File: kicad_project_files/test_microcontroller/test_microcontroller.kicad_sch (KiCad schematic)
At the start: 40 parts, among them J1 USB4510-03-1-A_REVA, SW1 SW_Push, SW2 SW_Push, SW3 SW_Push, SW4 SW_Push, SW5 SW_Push, SW6 SW_Push, SW7 SW_Push, SW8 SW_Push, SW9 SW_Push, U1 ATmega8U2-A, Y1 16mhz

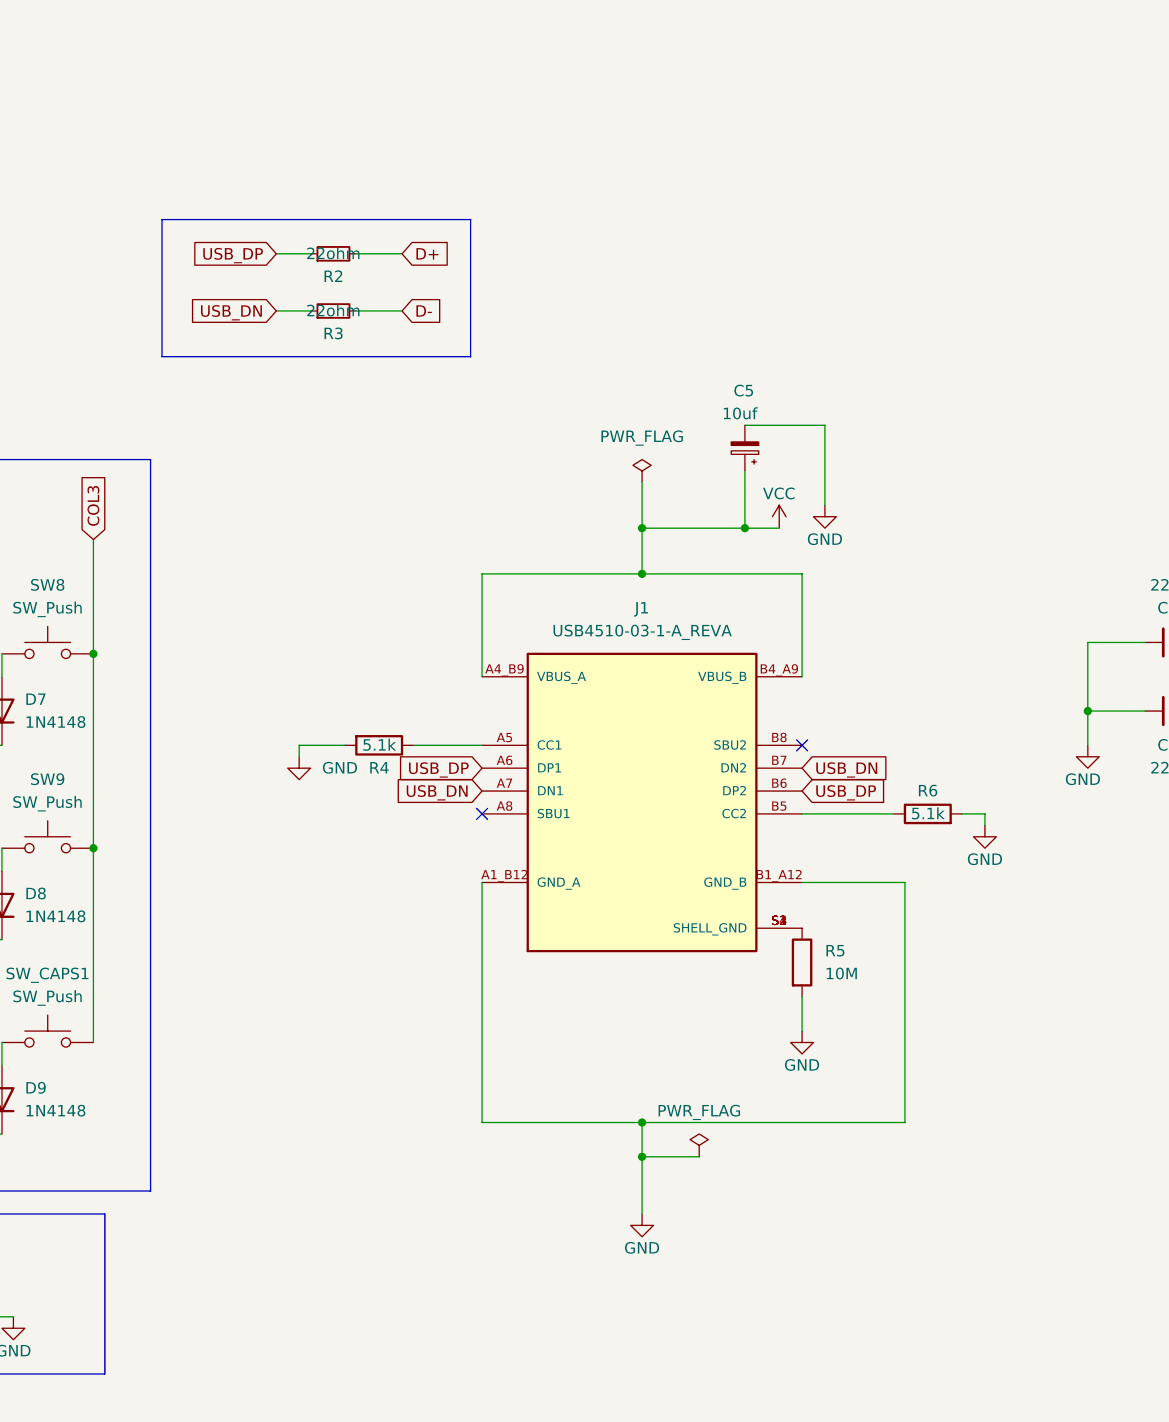
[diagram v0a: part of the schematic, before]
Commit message: Revert "Revert "Merge branch 'main' of https://github.com/Goochy12/Keych-and-Chong""
This reverts commit c8ae18377c4835621f54e74df08cb33c8008ec0a.
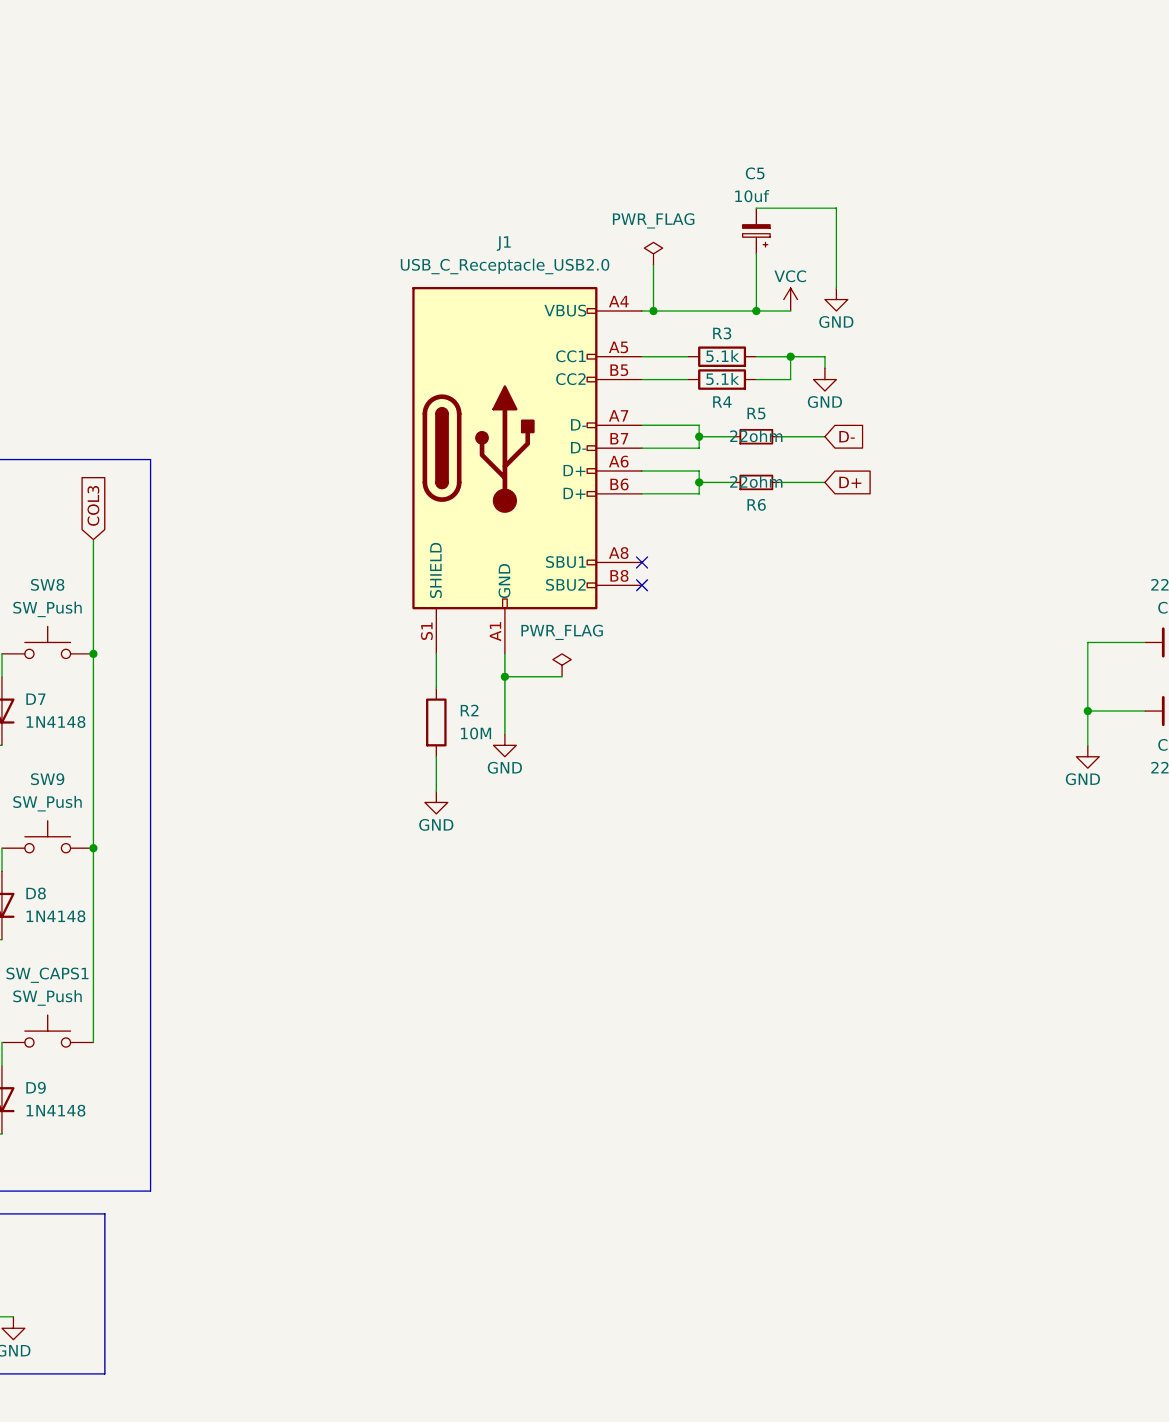
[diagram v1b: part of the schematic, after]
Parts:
- removed J1: USB4510-03-1-A_REVA, GCT_USB4510-03-1-A_REVA:GCT_USB4510-03-1-A_REVA, symbol USB4510-03-1-A_REVA:USB4510-03-1-A_REVA
- removed R2, R3: 22ohm, Resistor_THT:R_Axial_DIN0204_L3.6mm_D1.6mm_P5.08mm_Horizontal, symbol Device:R_Small
- removed R5: 10M, Resistor_THT:R_Axial_DIN0204_L3.6mm_D1.6mm_P5.08mm_Horizontal, symbol Device:R
- removed R6: 5.1k, Resistor_THT:R_Axial_DIN0204_L3.6mm_D1.6mm_P5.08mm_Horizontal, symbol Device:R
- added J1: USB_C_Receptacle_USB2.0, Connector_USB:USB_C_Receptacle_HRO_TYPE-C-31-M-12, symbol Connector:USB_C_Receptacle_USB2.0
- added R2: 10M, Resistor_THT:R_Axial_DIN0204_L3.6mm_D1.6mm_P5.08mm_Horizontal, symbol Device:R
- added R3: 5.1k, Resistor_THT:R_Axial_DIN0204_L3.6mm_D1.6mm_P5.08mm_Horizontal, symbol Device:R
- added R5, R6: 22ohm, Resistor_THT:R_Axial_DIN0204_L3.6mm_D1.6mm_P5.08mm_Horizontal, symbol Device:R_Small
- D_CAPS1: footprint CLA1A_SMD_LED:CLA1A-WKW-CXAYB153 -> LED_SMD:LED_Cree-PLCC4_3.2x2.8mm_CCW
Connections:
- net D+: now also R6.2
- net D-: now also R5.2
- net GND: now also J1.A1 (GND), J1.A12 (GND), J1.B1 (GND), J1.B12 (GND), R2.2, R3.2
- net VCC: now also J1.A4 (VBUS), J1.A9 (VBUS), J1.B4 (VBUS), J1.B9 (VBUS)
- net at R4.1: now also J1.B5 (CC2)
- new net: J1.A5 (CC1), R3.1
- new net: J1.A6 (D+), J1.B6 (D+), R6.1
- new net: J1.A7 (D-), J1.B7 (D-), R5.1
- new net: J1.S1 (SHIELD), R2.1

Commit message: Revert "Merge branch 'main' of https://github.com/Goochy12/Keych-and-Chong"
This reverts commit 16abbc7445c5651a73e155e9e96779087de1ba9e, reversing
changes made to 1815a7fd47ddf9f2f8e947e23bdaa21c8c5a7216.
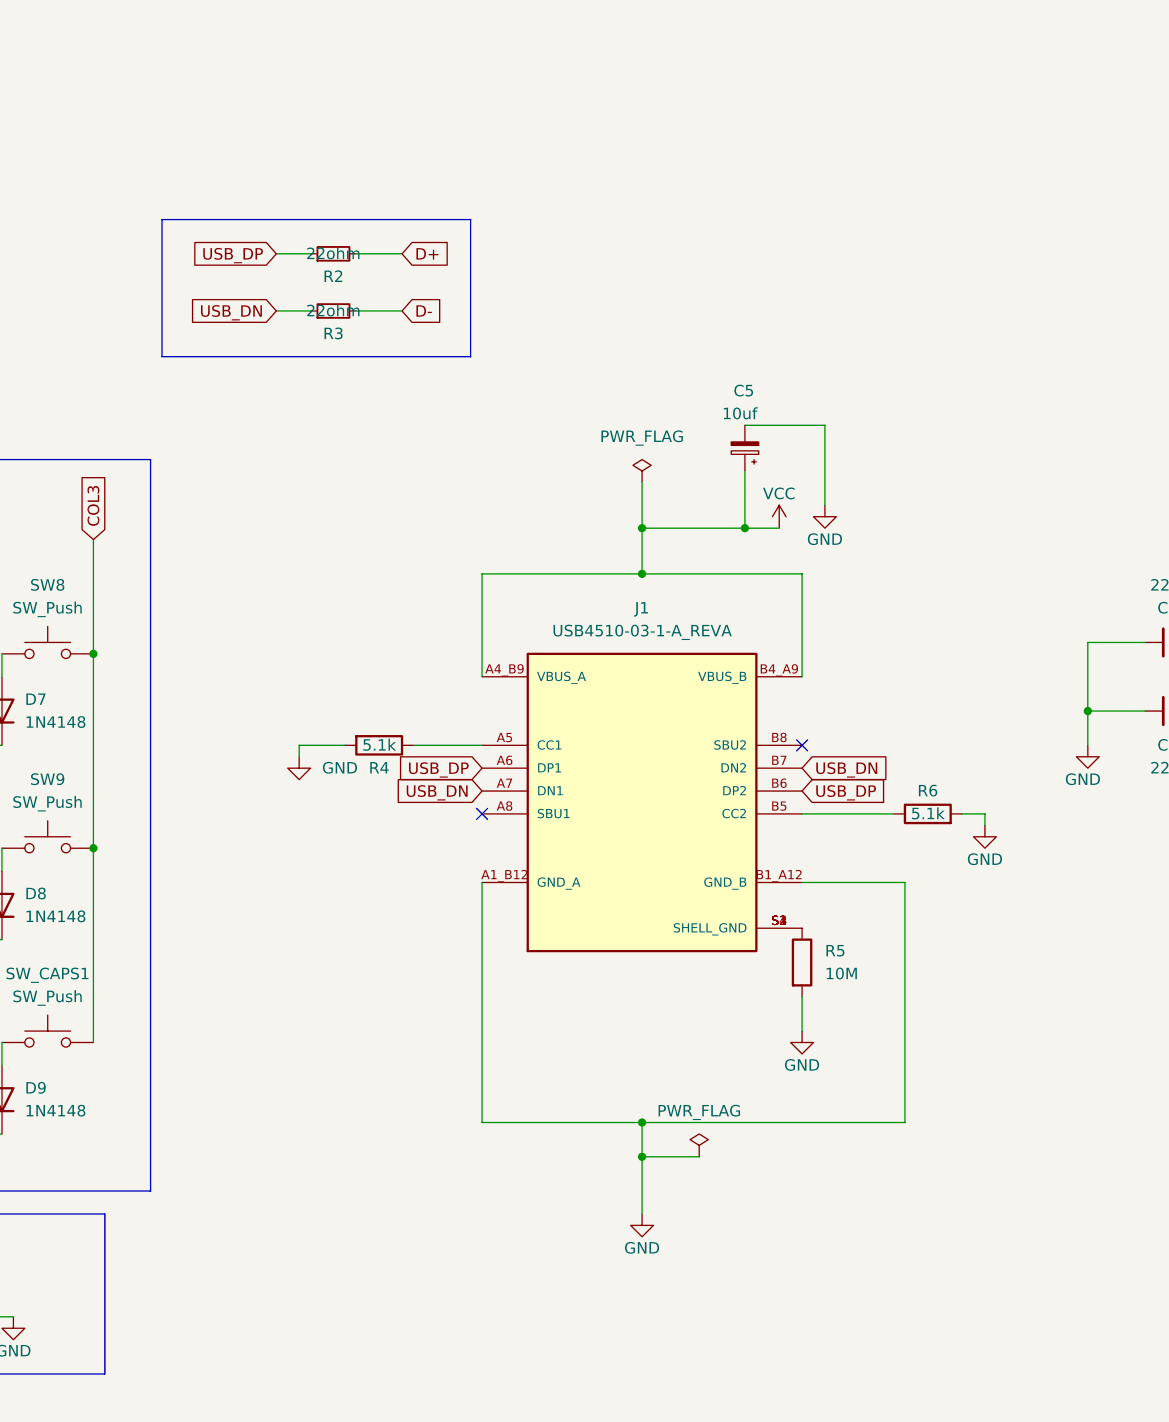
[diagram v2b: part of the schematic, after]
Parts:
- removed J1: USB_C_Receptacle_USB2.0, Connector_USB:USB_C_Receptacle_HRO_TYPE-C-31-M-12, symbol Connector:USB_C_Receptacle_USB2.0
- removed R2: 10M, Resistor_THT:R_Axial_DIN0204_L3.6mm_D1.6mm_P5.08mm_Horizontal, symbol Device:R
- removed R3: 5.1k, Resistor_THT:R_Axial_DIN0204_L3.6mm_D1.6mm_P5.08mm_Horizontal, symbol Device:R
- removed R5, R6: 22ohm, Resistor_THT:R_Axial_DIN0204_L3.6mm_D1.6mm_P5.08mm_Horizontal, symbol Device:R_Small
- added J1: USB4510-03-1-A_REVA, GCT_USB4510-03-1-A_REVA:GCT_USB4510-03-1-A_REVA, symbol USB4510-03-1-A_REVA:USB4510-03-1-A_REVA
- added R2, R3: 22ohm, Resistor_THT:R_Axial_DIN0204_L3.6mm_D1.6mm_P5.08mm_Horizontal, symbol Device:R_Small
- added R5: 10M, Resistor_THT:R_Axial_DIN0204_L3.6mm_D1.6mm_P5.08mm_Horizontal, symbol Device:R
- added R6: 5.1k, Resistor_THT:R_Axial_DIN0204_L3.6mm_D1.6mm_P5.08mm_Horizontal, symbol Device:R
- D_CAPS1: footprint LED_SMD:LED_Cree-PLCC4_3.2x2.8mm_CCW -> CLA1A_SMD_LED:CLA1A-WKW-CXAYB153
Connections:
- net D+: now also R2.2
- net D-: now also R3.2
- net GND: now also J1.A1_B12 (GND_A), J1.B1_A12 (GND_B), R5.2, R6.2
- net VCC: now also J1.A4_B9 (VBUS_A), J1.B4_A9 (VBUS_B)
- net at R4.1: now also J1.A5 (CC1)
- new net: J1.B5 (CC2), R6.1
- new net: J1.S1 (SHELL_GND), J1.S2 (SHELL_GND), J1.S3 (SHELL_GND), J1.S4 (SHELL_GND), R5.1
- new net USB_DN: J1.A7 (DN1), J1.B7 (DN2), R3.1
- new net USB_DP: J1.A6 (DP1), J1.B6 (DP2), R2.1

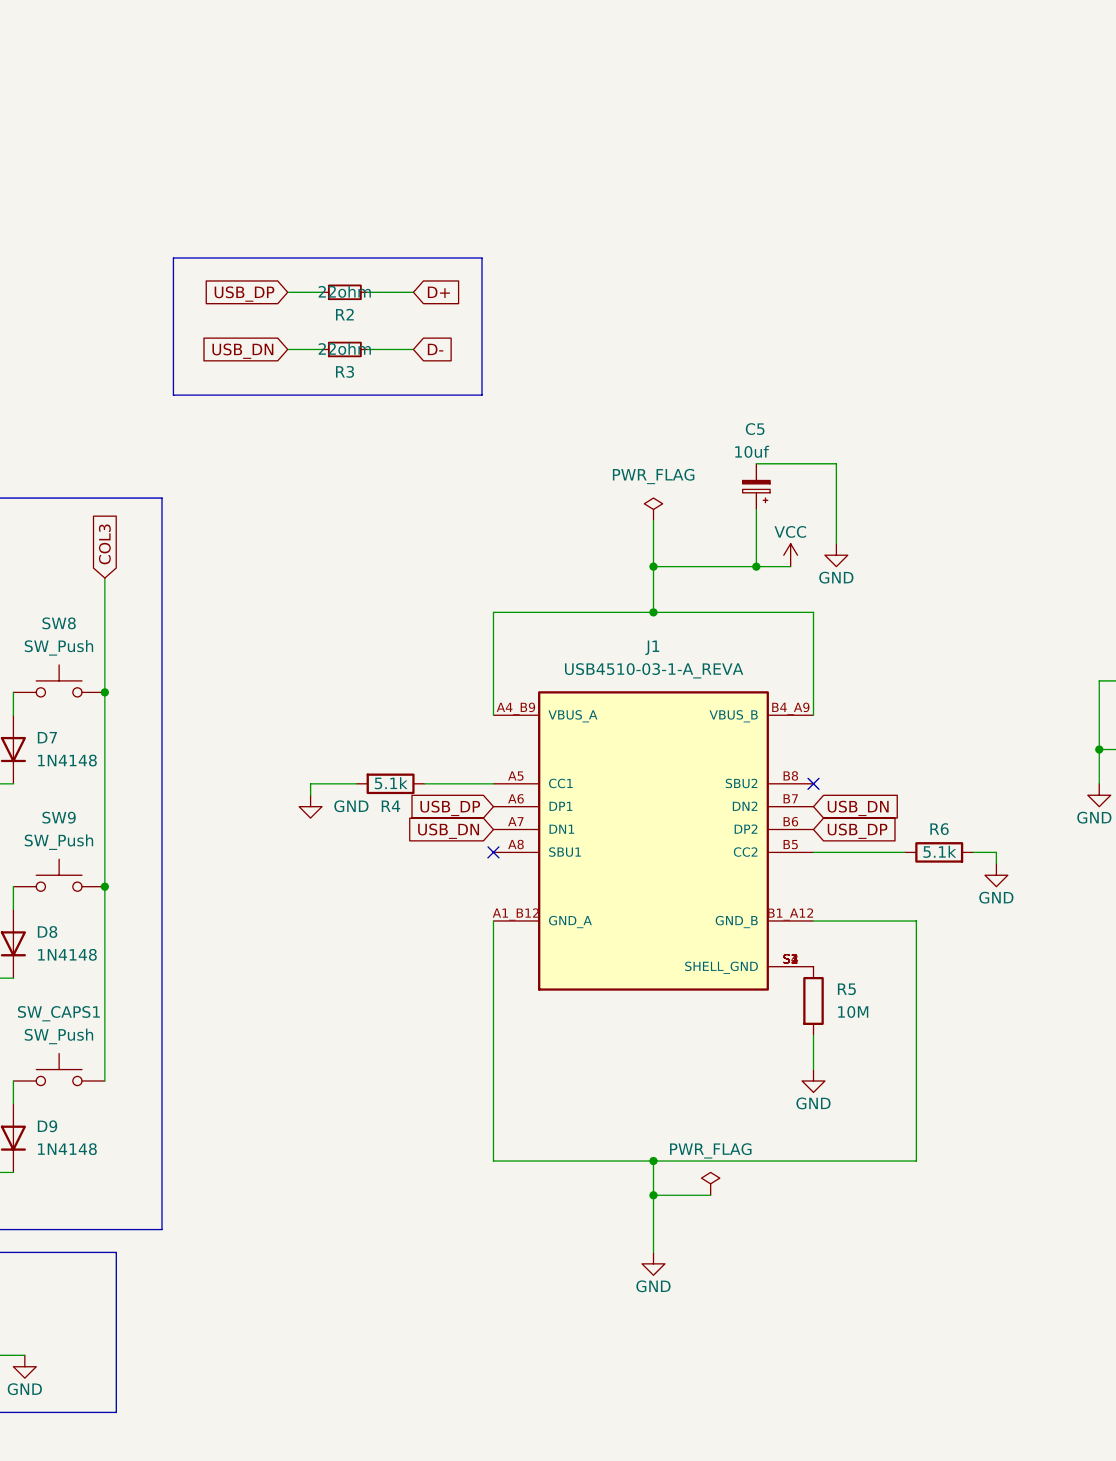
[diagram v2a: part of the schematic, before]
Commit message: Revert "Merge branch 'main' of https://github.com/Goochy12/Keych-and-Chong"
This reverts commit 89a84faf58301de3235cbf20de78d9bc04a2e137, reversing
changes made to 8f87e55d37906a6161fcb491ec761d32a82a7e61.
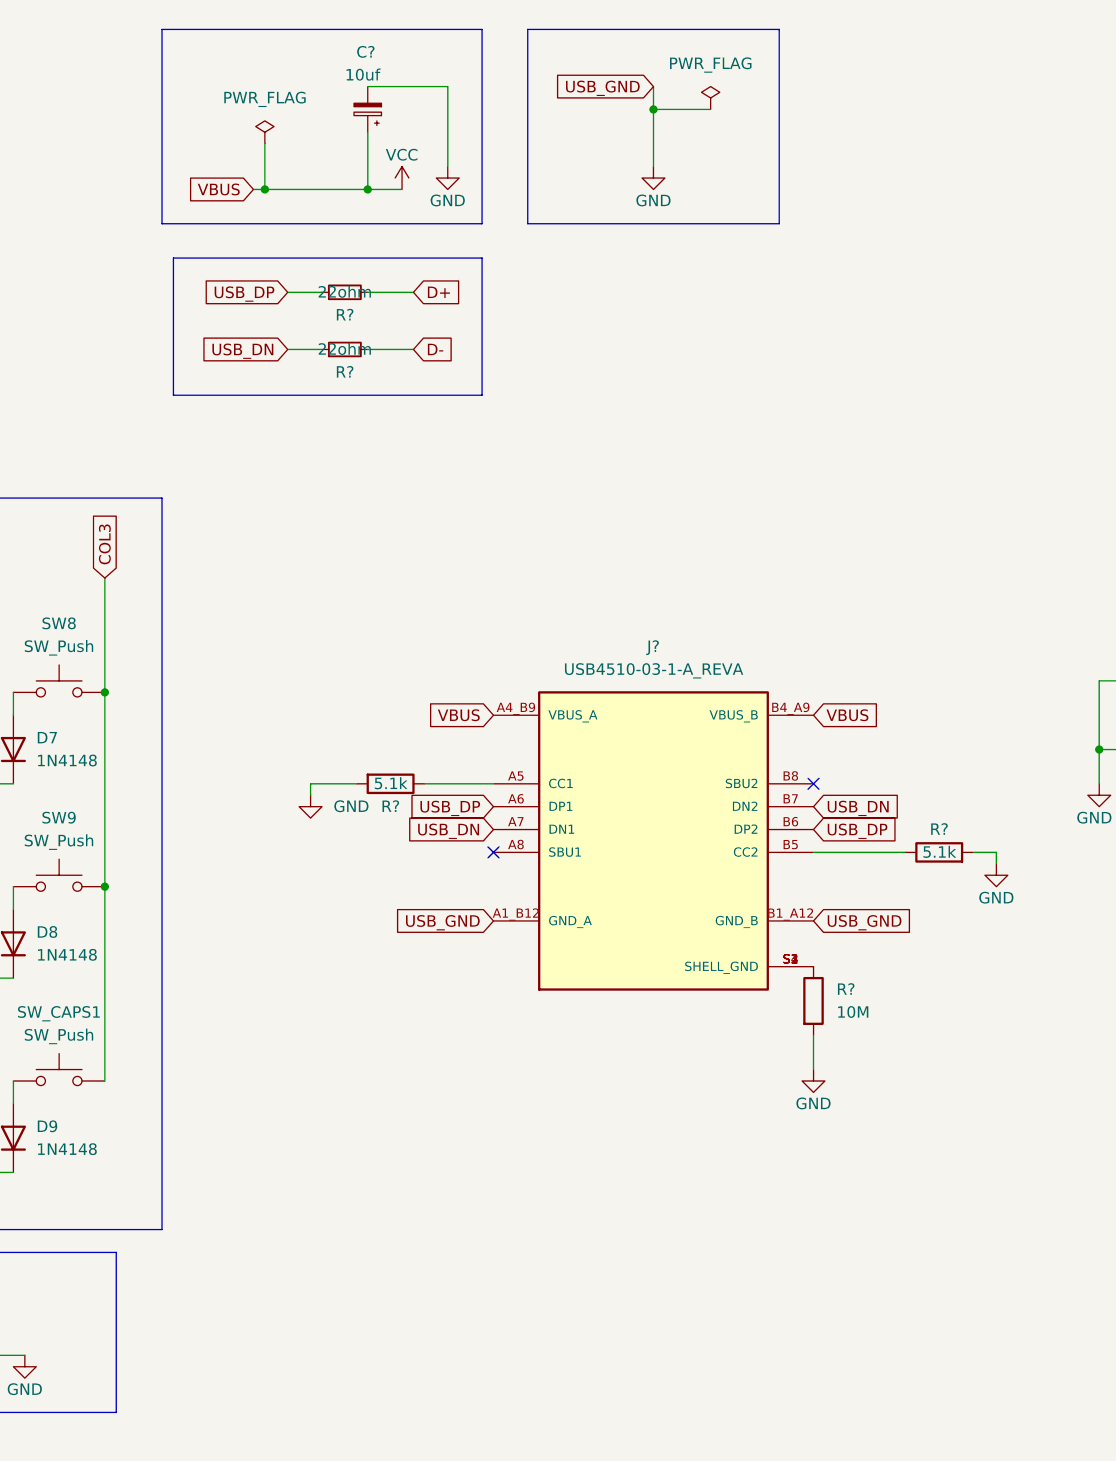
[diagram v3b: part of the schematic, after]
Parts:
- removed C5: 10uf, Capacitor_THT:CP_Radial_D4.0mm_P1.50mm, symbol Device:C_Polarized_Small
- added C?: 10uf, Capacitor_THT:CP_Radial_D4.0mm_P1.50mm, symbol Device:C_Polarized_Small
- D_CAPS1: footprint CLA1A_SMD_LED:CLA1A-WKW-CXAYB153 -> LED_SMD:LED_Cree-PLCC4_3.2x2.8mm_CCW
- J?: renamed from J1; footprint GCT_USB4510-03-1-A_REVA:GCT_USB4510-03-1-A_REVA -> GCT_USB4510-03-1-A_REVA
- renumbered R4 to R?, R5 to R?, R6 to R?, R2 to R?, R3 to R?
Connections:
- net GND: now also C?.2
- net VCC: now also C?.1
